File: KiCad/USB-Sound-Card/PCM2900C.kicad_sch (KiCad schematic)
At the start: 21 parts, among them J101 USB_C_Receptacle_USB2.0, J102 AudioJack3, U101 PCM2900C, Y1 12MHz 18pF

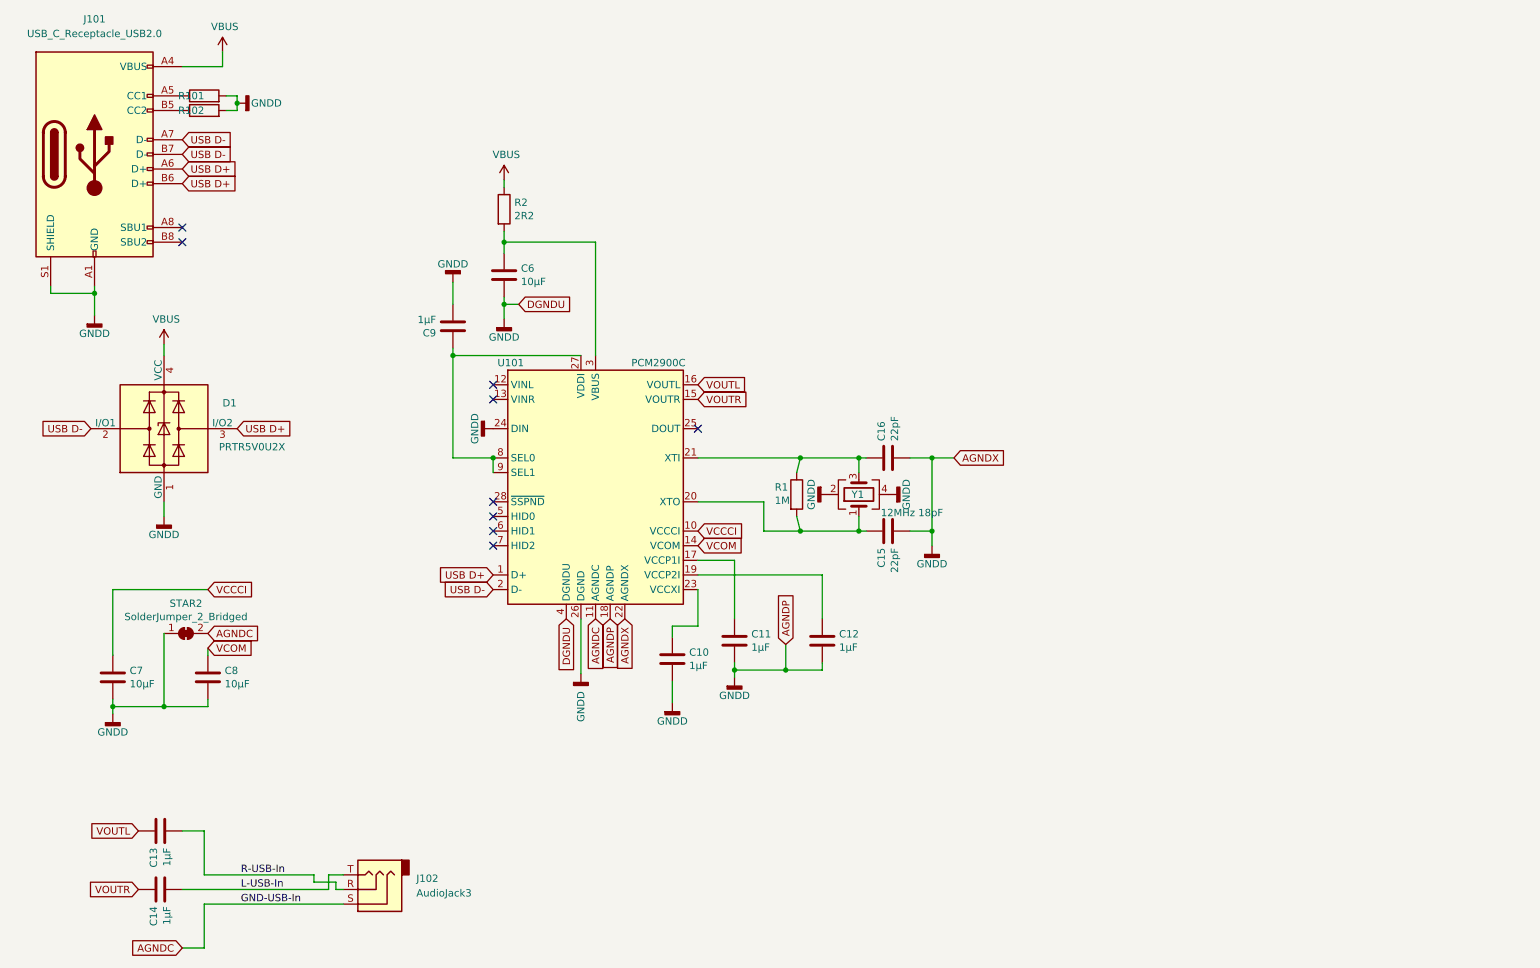
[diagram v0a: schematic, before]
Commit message: added some amps, may change
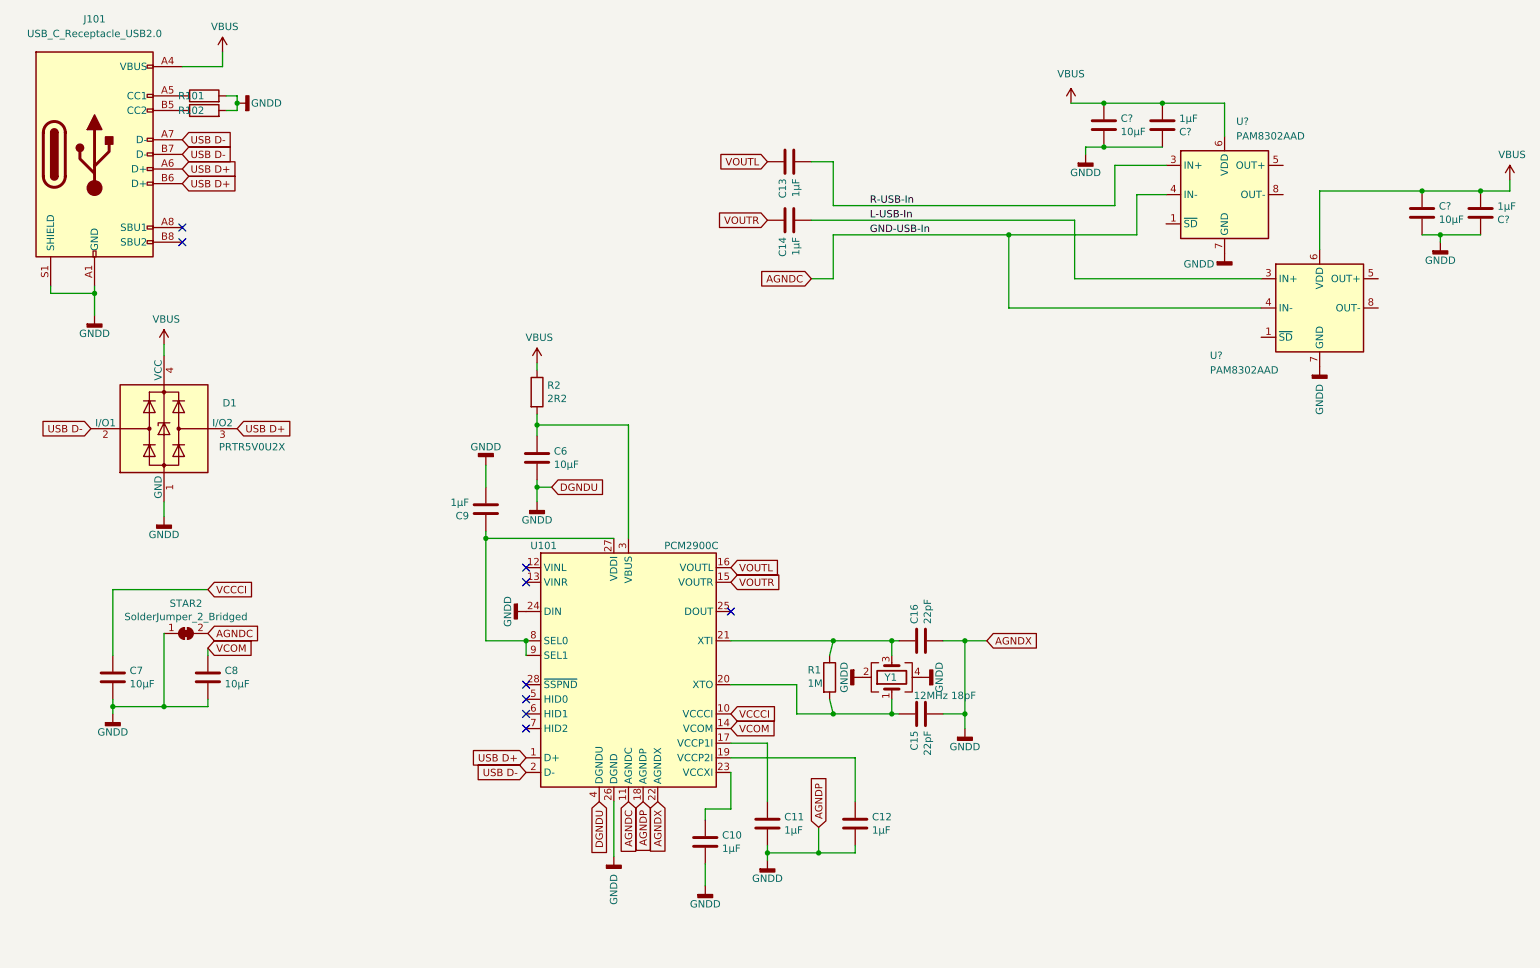
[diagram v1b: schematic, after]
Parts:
- removed J102: AudioJack3, Connector_Audio:Jack_3.5mm_CUI_SJ1-3523N_Horizontal, symbol Connector:AudioJack3
- added C? (x2): 10µF, Capacitor_SMD:C_0402_1005Metric, symbol Device:C
- added C? (x2): 1µF, Capacitor_SMD:C_0402_1005Metric, symbol Device:C
- added U? (x2): PAM8302AAD, Package_SO:Diodes_SO-8EP, symbol Amplifier_Audio:PAM8302AAD
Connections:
- net AGNDC: now also U?.4 (IN-), U?.4 (IN-)
- net GNDD: now also C?.1, C?.1, C?.2, C?.2, U?.7 (GND), U?.7 (GND)
- net L-USB-In: now also U?.3 (IN+)
- net R-USB-In: now also U?.3 (IN+)
- net VBUS: now also C?.1, C?.1, C?.2, C?.2, U?.6 (VDD), U?.6 (VDD)
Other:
- moved on the sheet: C10, C11, C12, C13, C14, C15, C16, C6, C9, R1, R2, U101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
